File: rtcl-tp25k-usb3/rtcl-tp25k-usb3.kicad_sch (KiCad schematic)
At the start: 76 parts, among them J1 ZX360D-B-10P(30), J10 SSQ-106-02-F-D-RA, J2 0525592253, J3 BTB-DF40C-60DS-0.4V(51), J4 DF40C-60DS-0.4V(51), J5 JTAG, U1 FT601Q, U2 TPD4E05U06DQA, U3 USBLC6-2P6, U4 TPS62826DMQR, U5 PCA9306DC, X1 ABM8-30.000MHZ-D1X-T

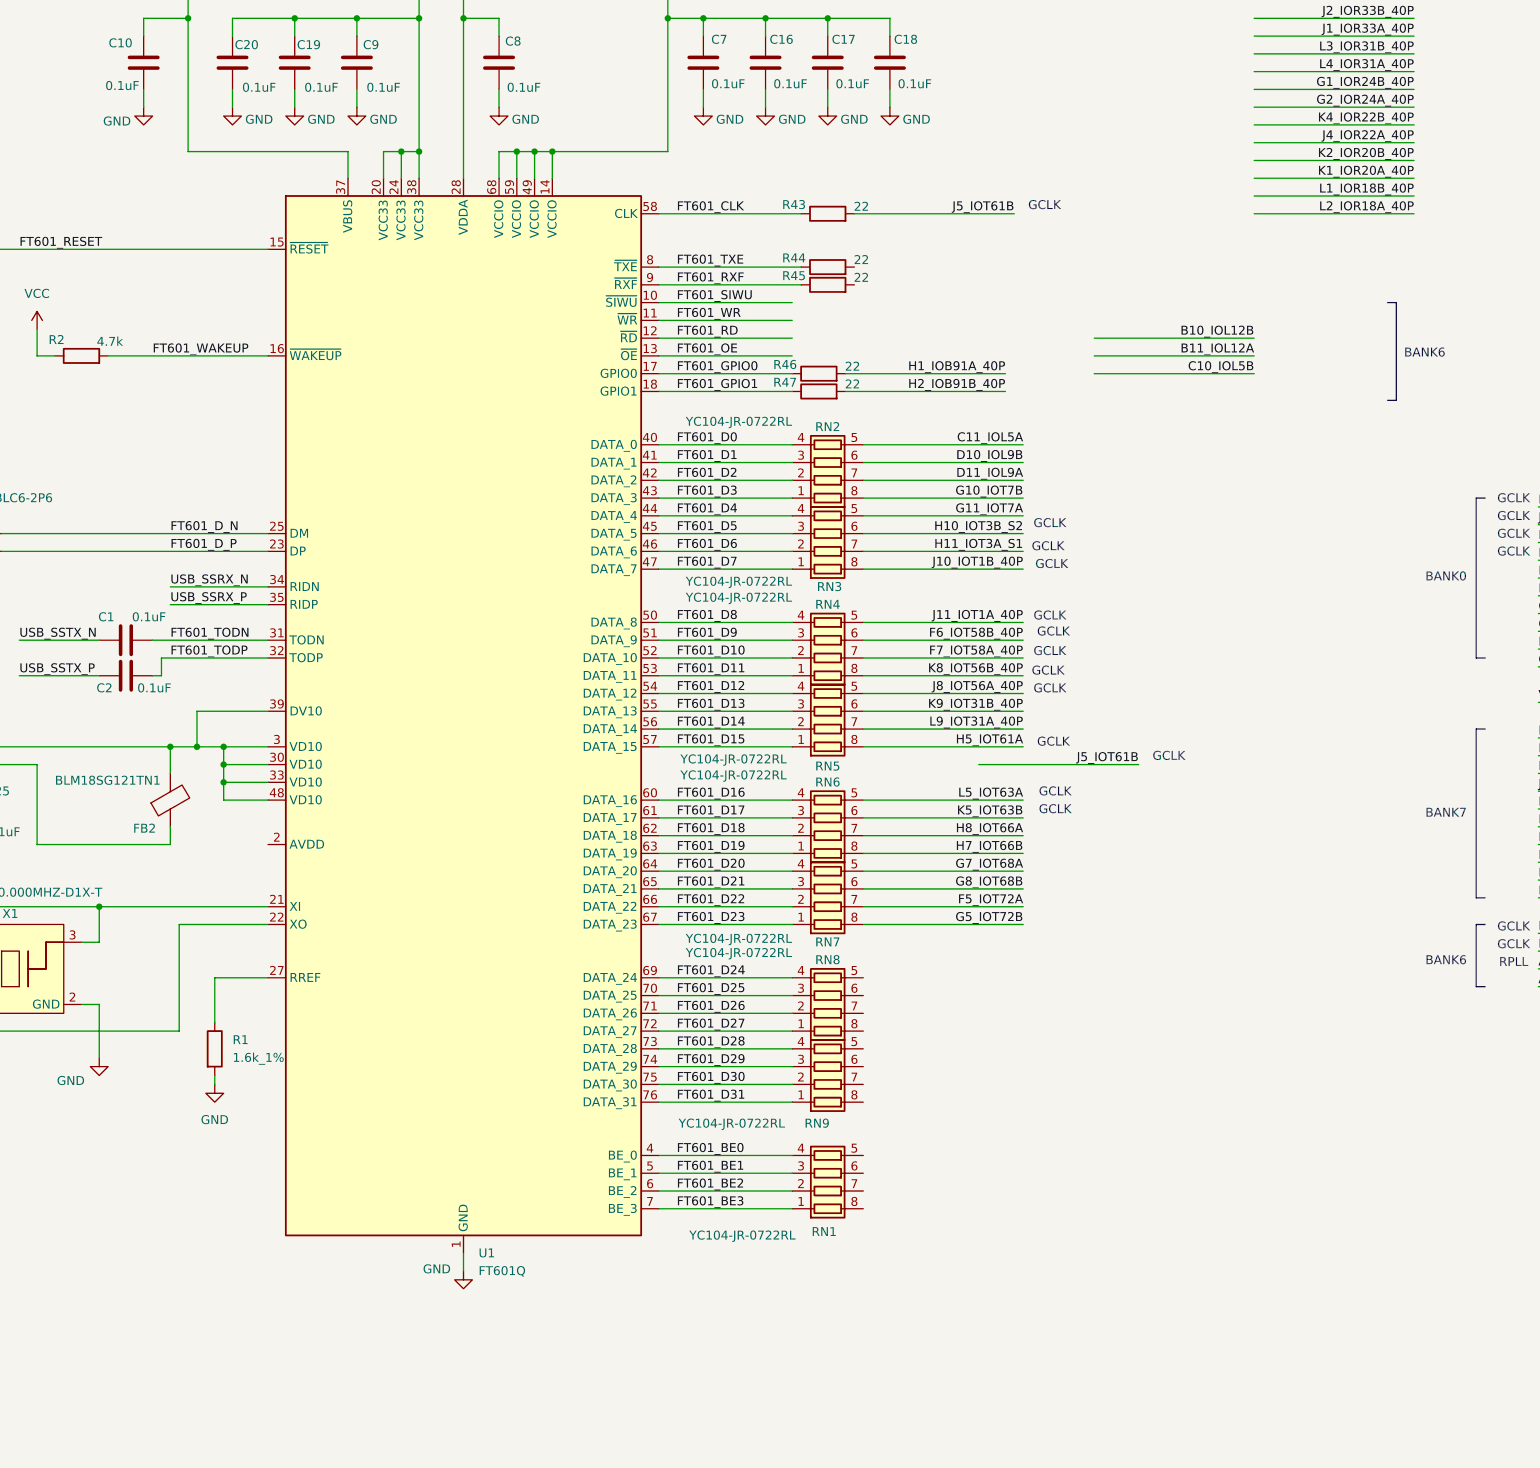
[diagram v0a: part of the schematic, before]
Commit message: WIP
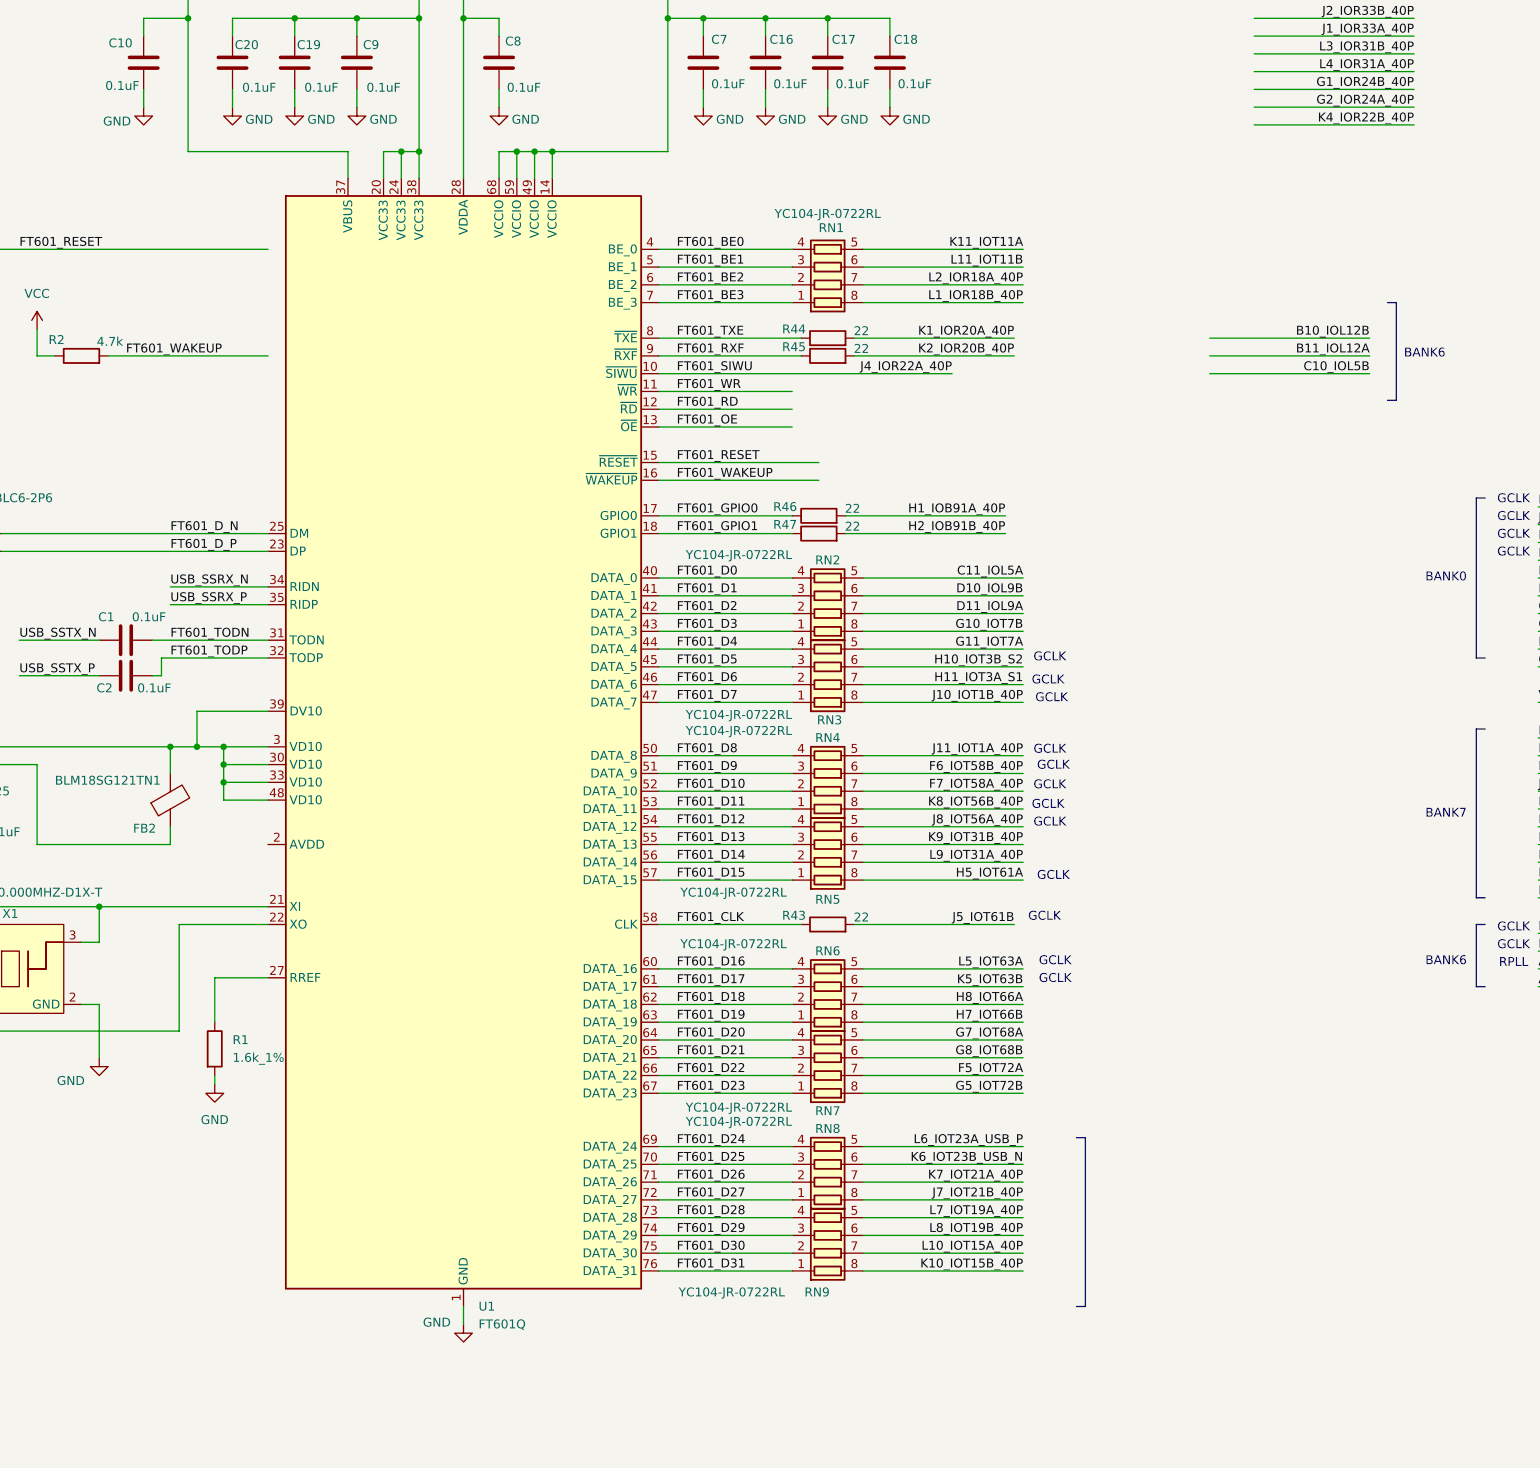
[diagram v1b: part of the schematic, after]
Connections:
- net J4_IOR22A_40P is gone; now on net FT601_SIWU: J4.14 (Pin_14)
- net J7_IOT21B_40P: now also RN8.8 (R1.2)
- net K10_IOT15B_40P: now also RN9.8 (R1.2)
- net K11_IOT11A: now also RN1.5 (R4.2)
- net K1_IOR20A_40P: now also R44.2
- net K2_IOR20B_40P: now also R45.2
- net K6_IOT23B_USB_N: now also RN8.6 (R3.2)
- net K7_IOT21A_40P: now also RN8.7 (R2.2)
- net L10_IOT15A_40P: now also RN9.7 (R2.2)
- net L11_IOT11B: now also RN1.6 (R3.2)
- net L1_IOR18B_40P: now also RN1.8 (R1.2)
- net L2_IOR18A_40P: now also RN1.7 (R2.2)
- net L6_IOT23A_USB_P: now also RN8.5 (R4.2)
- net L7_IOT19A_40P: now also RN9.5 (R4.2)
- net L8_IOT19B_40P: now also RN9.6 (R3.2)
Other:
- moved on the sheet: R43, R44, R45, R46, R47, RN1, RN2, RN3, RN4, RN5, RN6, RN7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
